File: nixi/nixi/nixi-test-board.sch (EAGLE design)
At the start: 18 parts, among them IC1 7805T, IC2-ATTINY85 TINY15LP, Q1 MRF136, Q2 2N6107, Q3 BC238

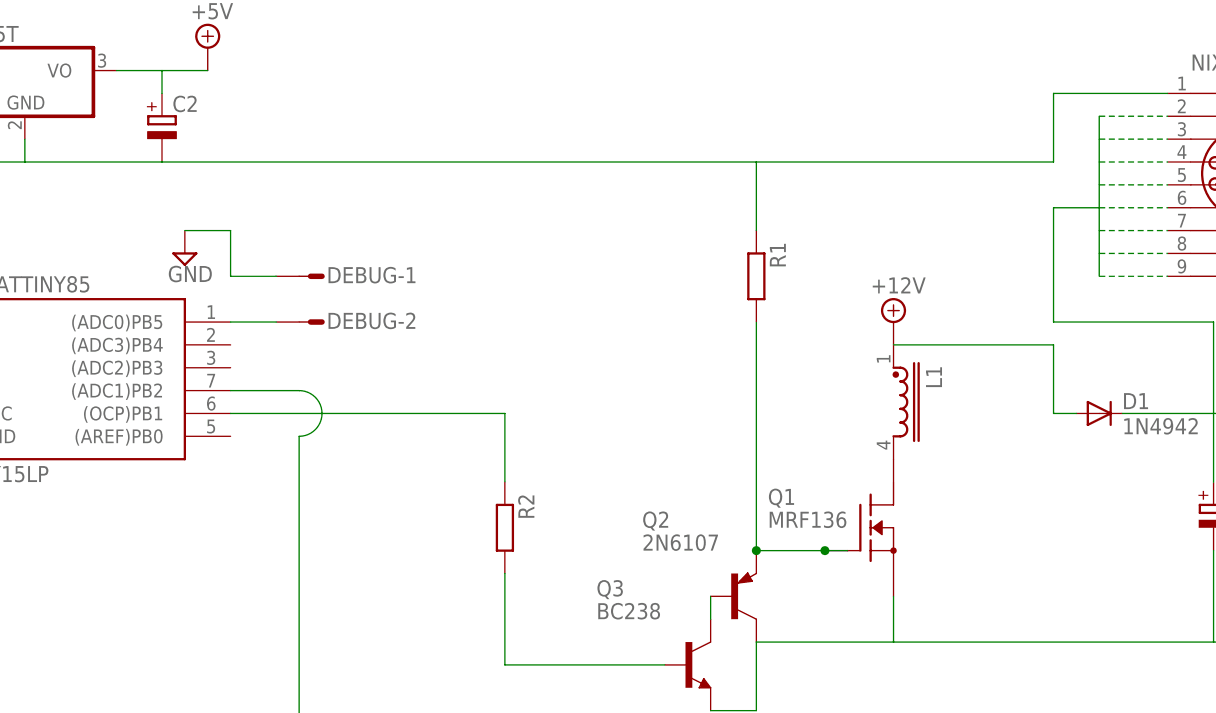
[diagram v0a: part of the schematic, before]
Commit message: reg save
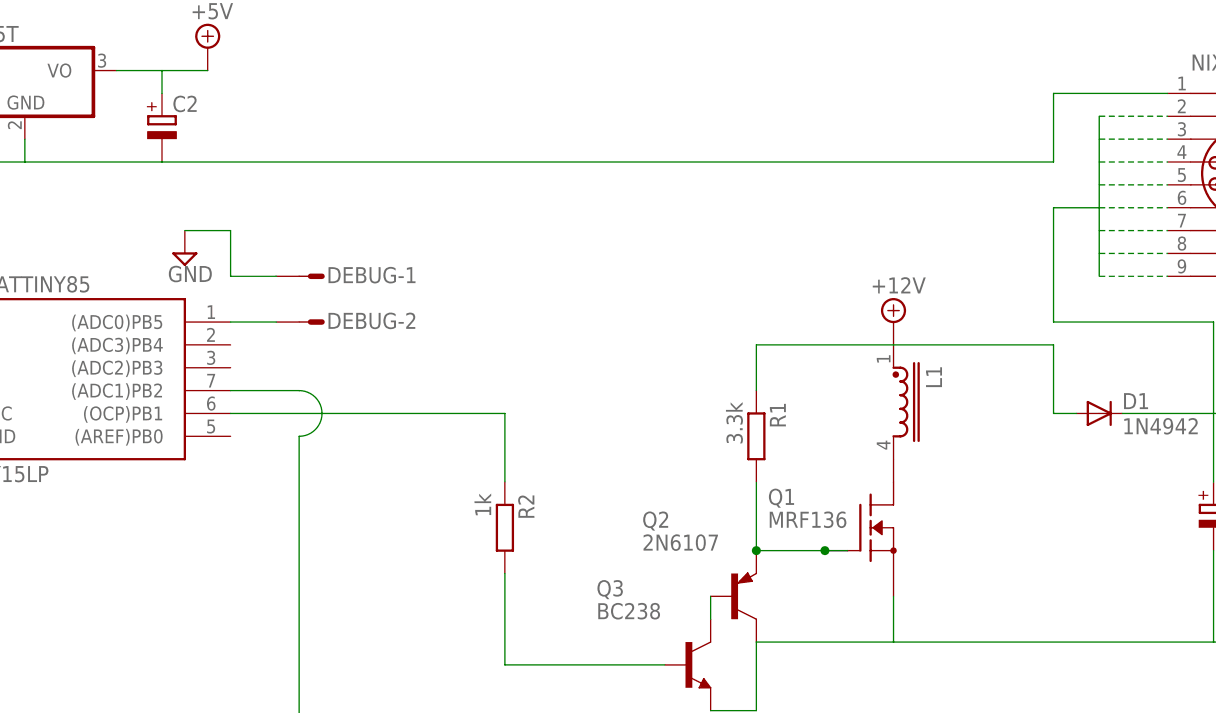
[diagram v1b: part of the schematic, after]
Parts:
- R1: value (none) -> 3.3k
- R2: value (none) -> 1k
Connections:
- net +12V: now also R1.1
- net GND: no longer R1.1
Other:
- moved on the sheet: R1
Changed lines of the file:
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@@
 <part name="RV1" library="resistor" deviceset="R-TRIMM" device="4G/J"/>
 <part name="Q2" library="transistor-pnp" deviceset="2N6107" device=""/>
-<part name="R1" library="resistor" deviceset="R-EU_" device="0207/5V"/>
-<part name="R2" library="resistor" deviceset="R-EU_" device="0207/5V"/>
+<part name="R1" library="resistor" deviceset="R-EU_" device="0207/5V" value="3.3k"/>
+<part name="R2" library="resistor" deviceset="R-EU_" device="0207/5V" value="1k"/>
 <part name="Q3" library="transistor-npn" deviceset="BC238" device=""/>
 </parts>
@@
 <instance part="RV1" gate="G$1" x="170.18" y="25.4"/>
 <instance part="Q2" gate="G$1" x="96.52" y="22.86"/>
-<instance part="R1" gate="G$1" x="99.06" y="58.42" rot="R270"/>
+<instance part="R1" gate="G$1" x="99.06" y="40.64" rot="R270"/>
 <instance part="R2" gate="G$1" x="71.12" y="30.48" rot="R270"/>
 <instance part="Q3" gate="G$1" x="91.44" y="15.24"/>
@@
 <wire x1="17.78" y1="71.12" x2="17.78" y2="73.66" width="0.1524" layer="91"/>
 <wire x1="17.78" y1="71.12" x2="33.02" y2="71.12" width="0.1524" layer="91"/>
-<wire x1="33.02" y1="71.12" x2="99.06" y2="71.12" width="0.1524" layer="91"/>
-<wire x1="99.06" y1="71.12" x2="132.08" y2="71.12" width="0.1524" layer="91"/>
+<wire x1="33.02" y1="71.12" x2="132.08" y2="71.12" width="0.1524" layer="91"/>
 <wire x1="132.08" y1="71.12" x2="132.08" y2="78.74" width="0.1524" layer="91"/>
 <pinref part="NIXI-SOCKET" gate="G$1" pin="1"/>
@@
 <pinref part="C3" gate="G$1" pin="-"/>
 <pinref part="GND" gate="-1" pin="S"/>
-<pinref part="R1" gate="G$1" pin="1"/>
-<wire x1="99.06" y1="71.12" x2="99.06" y2="63.5" width="0.1524" layer="91"/>
 </segment>
 <segment>
@@
 <pinref part="D1" gate="1" pin="A"/>
 <wire x1="132.08" y1="43.18" x2="134.62" y2="43.18" width="0.1524" layer="91"/>
+<wire x1="114.3" y1="50.8" x2="99.06" y2="50.8" width="0.1524" layer="91"/>
+<pinref part="R1" gate="G$1" pin="1"/>
+<wire x1="99.06" y1="50.8" x2="99.06" y2="45.72" width="0.1524" layer="91"/>
 </segment>
 </net>
@@
 <wire x1="99.06" y1="27.94" x2="106.68" y2="27.94" width="0.1524" layer="91"/>
 <pinref part="R1" gate="G$1" pin="2"/>
-<wire x1="99.06" y1="53.34" x2="99.06" y2="27.94" width="0.1524" layer="91"/>
+<wire x1="99.06" y1="35.56" x2="99.06" y2="27.94" width="0.1524" layer="91"/>
 <pinref part="Q2" gate="G$1" pin="E"/>
 <junction x="99.06" y="27.94"/>
